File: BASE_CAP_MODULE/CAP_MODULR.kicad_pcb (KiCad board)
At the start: 2 copper layers, 42.1 x 30.4 mm, 8 parts

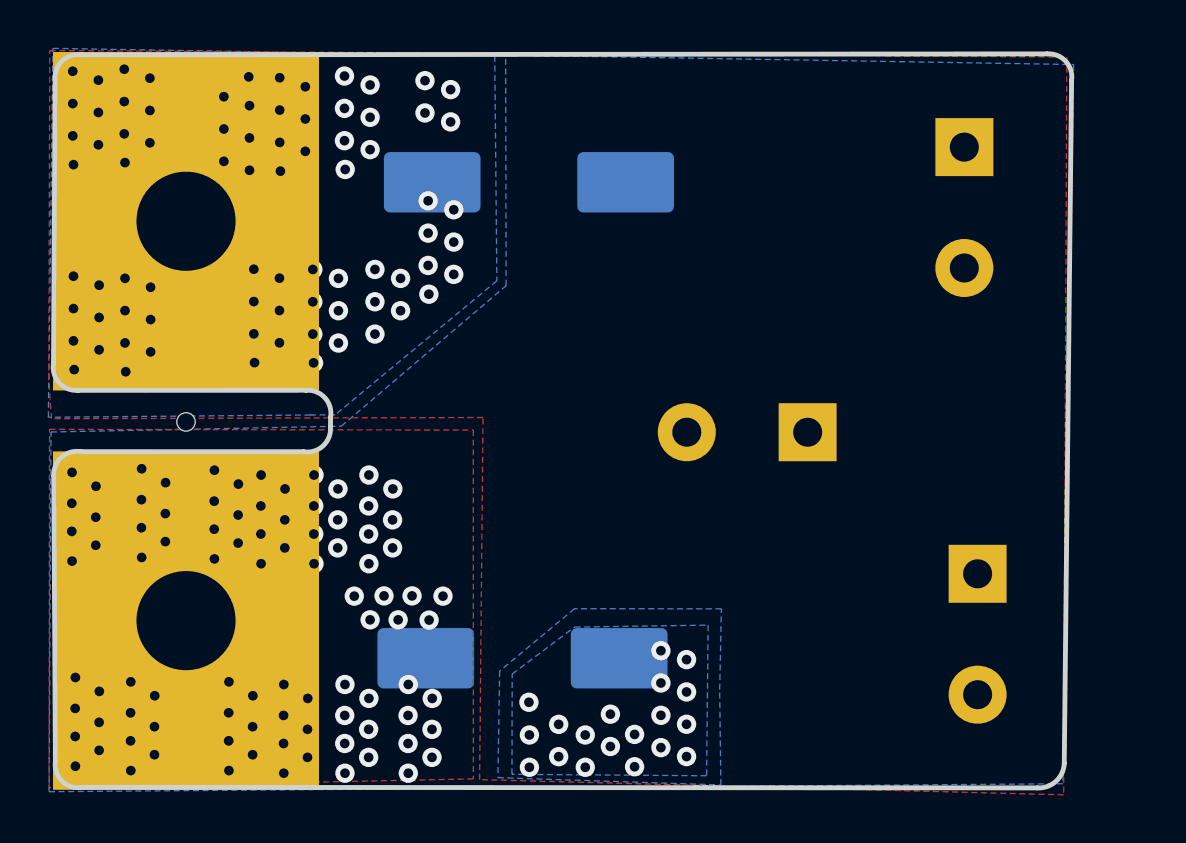
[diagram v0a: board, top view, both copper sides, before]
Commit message: Log
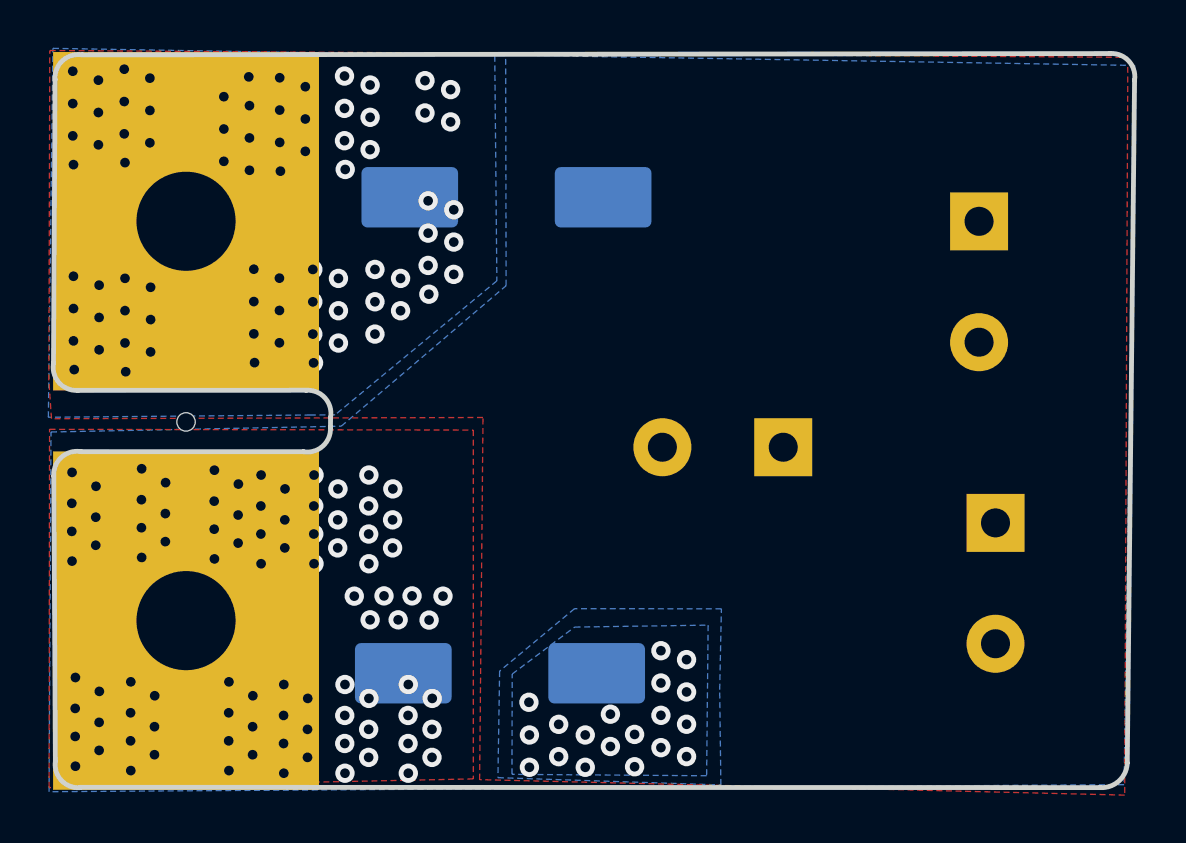
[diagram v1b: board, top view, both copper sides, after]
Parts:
- moved REF** 3.13 mm to (160.8, 88.6)
- moved REF** 2.23 mm to (161.4, 101.1)
- moved REF** 1.19 mm to (152.7, 98.0)
- moved REF** 1.12 mm to (141.2, 87.6)
- moved REF** 1.12 mm to (140.9, 107.3)
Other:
- board size 42.1 x 30.4 mm -> 44.7 x 30.4 mm
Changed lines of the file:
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@@
   )
   (footprint "Capacitor_SMD:CP_Elec_10x10" (layer "B.Cu")
-    (at 142.13 87.01)
+    (at 141.2 87.63)
     (descr "SMD capacitor, aluminum electrolytic, Nichicon, 10.0x10.0mm")
     (tags "capacitor electrolytic")
@@
   )
   (footprint "Capacitor_SMD:CP_Elec_10x10" (layer "B.Cu")
-    (at 141.8625 106.7 180)
+    (at 140.9325 107.32 180)
     (descr "SMD capacitor, aluminum electrolytic, Nichicon, 10.0x10.0mm")
     (tags "capacitor electrolytic")
@@
   )
   (footprint "Capacitor_THT:CP_Radial_D12.5mm_P5.00mm" (layer "B.Cu")
-    (at 153.66 97.35 180)
+    (at 152.65 97.97 180)
     (descr "CP, Radial series, Radial, pin pitch=5.00mm, , diameter=12.5mm, Electrolytic Capacitor")
     (tags "CP Radial series Radial pin pitch 5.00mm  diameter 12.5mm Electrolytic Capacitor")
@@
   )
   (footprint "Capacitor_THT:CP_Radial_D12.5mm_P5.00mm" (layer "B.Cu")
-    (at 160.69 103.206041 -90)
+    (at 161.43 101.1 -90)
     (descr "CP, Radial series, Radial, pin pitch=5.00mm, , diameter=12.5mm, Electrolytic Capacitor")
     (tags "CP Radial series Radial pin pitch 5.00mm  diameter 12.5mm Electrolytic Capacitor")
@@
   )
   (footprint "Capacitor_THT:CP_Radial_D12.5mm_P5.00mm" (layer "B.Cu")
-    (at 160.14 85.556041 -90)
+    (at 160.75 88.626041 -90)
     (descr "CP, Radial series, Radial, pin pitch=5.00mm, , diameter=12.5mm, Electrolytic Capacitor")
     (tags "CP Radial series Radial pin pitch 5.00mm  diameter 12.5mm Electrolytic Capacitor")
@@
   )
   (gr_line (start 132.799869 98.15583) (end 123.595221 98.15313) (layer "Edge.Cuts") (width 0.2))
-  (gr_line (start 123.551544 112.037739) (end 163.154244 112.063092) (layer "Edge.Cuts") (width 0.2))
+  (gr_line (start 123.551544 112.037739) (end 165.76 112.05) (layer "Edge.Cuts") (width 0.2))
   (gr_arc (start 122.529596 82.763091) (mid 122.839367 81.977705) (end 123.649596 81.740391) (layer "Edge.Cuts") (width 0.2))
   (gr_line (start 133.925221 96.73313) (end 133.919869 97.14583) (layer "Edge.Cuts") (width 0.2))
@@
   (gr_arc (start 133.919869 97.14583) (mid 133.605334 97.923029) (end 132.799869 98.15583) (layer "Edge.Cuts") (width 0.2))
   (gr_line (start 122.475221 99.16313) (end 122.541544 110.943091) (layer "Edge.Cuts") (width 0.2))
-  (gr_arc (start 164.274244 111.043092) (mid 163.930002 111.789992) (end 163.154244 112.063092) (layer "Edge.Cuts") (width 0.2))
+  (gr_arc (start 166.88 111.03) (mid 166.535763 111.776939) (end 165.76 112.05) (layer "Edge.Cuts") (width 0.2))
   (gr_arc (start 123.472521 95.617778) (mid 122.695322 95.303243) (end 122.462521 94.497778) (layer "Edge.Cuts") (width 0.2))
   (gr_line (start 122.462521 94.510478) (end 122.529596 82.763091) (layer "Edge.Cuts") (width 0.2))
-  (gr_line (start 123.649596 81.740391) (end 163.554244 81.698444) (layer "Edge.Cuts") (width 0.2))
+  (gr_line (start 123.649596 81.740391) (end 166.16 81.685352) (layer "Edge.Cuts") (width 0.2))
   (gr_arc (start 122.475221 99.16313) (mid 122.789756 98.385931) (end 123.595221 98.15313) (layer "Edge.Cuts") (width 0.2))
   (gr_arc (start 123.551544 112.052939) (mid 122.784177 111.747709) (end 122.541544 110.958291) (layer "Edge.Cuts") (width 0.2))
-  (gr_line (start 164.576944 82.793092) (end 164.274244 111.043092) (layer "Edge.Cuts") (width 0.2))
-  (gr_arc (start 163.554244 81.698444) (mid 164.329602 81.999133) (end 164.576944 82.793092) (layer "Edge.Cuts") (width 0.2))
+  (gr_line (start 167.1827 82.78) (end 166.88 111.03) (layer "Edge.Cuts") (width 0.2))
+  (gr_arc (start 166.16 81.685352) (mid 166.935317 81.986042) (end 167.1827 82.78) (layer "Edge.Cuts") (width 0.2))
   (gr_line (start 123.472521 95.617778) (end 132.915221 95.61313) (layer "Edge.Cuts") (width 0.2))
   (via (at 135.56 85.66) (size 0.8) (drill 0.4) (layers "F.Cu" "B.Cu") (free) (net 1))
@@
     (polygon
       (pts
-        (xy 164.38 81.83)
-        (xy 164.25 112.35)
+        (xy 166.903693 81.84075)
+        (xy 166.773693 112.36075)
         (xy 140.09 111.72)
         (xy 140.23 96.74)
@@
     (polygon
       (pts
-        (xy 164.66 82.14)
-        (xy 164.22 111.89)
+        (xy 167.188297 82.177393)
+        (xy 166.748297 111.927393)
         (xy 122.28 112.22)
         (xy 122.36 97.34)
